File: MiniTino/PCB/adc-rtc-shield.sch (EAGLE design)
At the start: 51 parts, among them IC1 TLC2543, IC2 RV_3049_C2

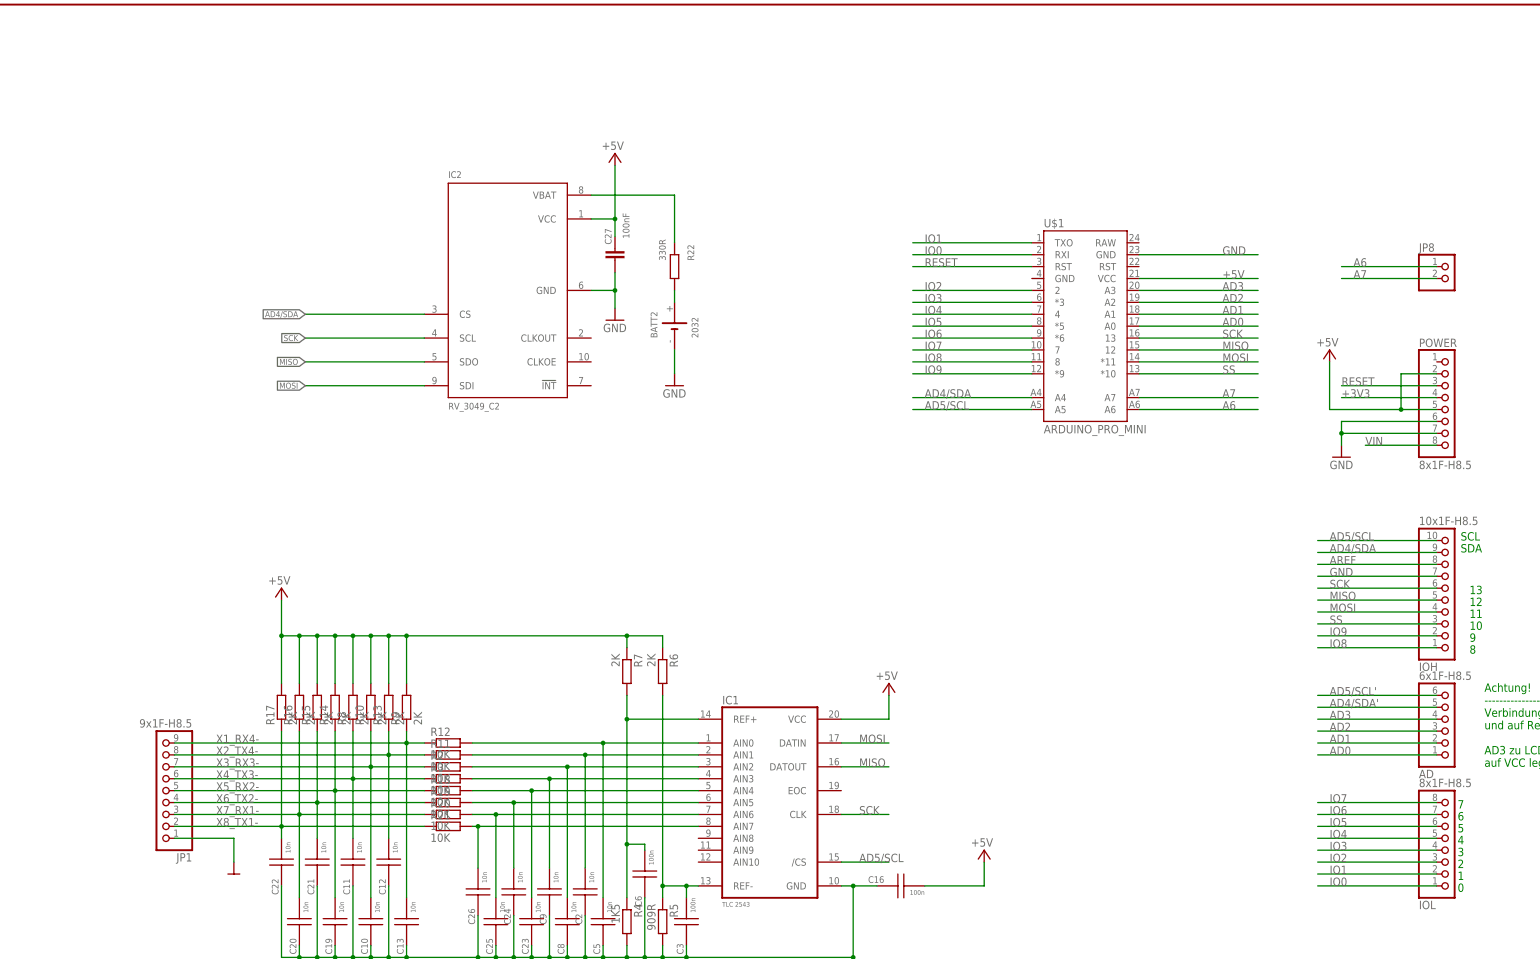
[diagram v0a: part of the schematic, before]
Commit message: Start routing.
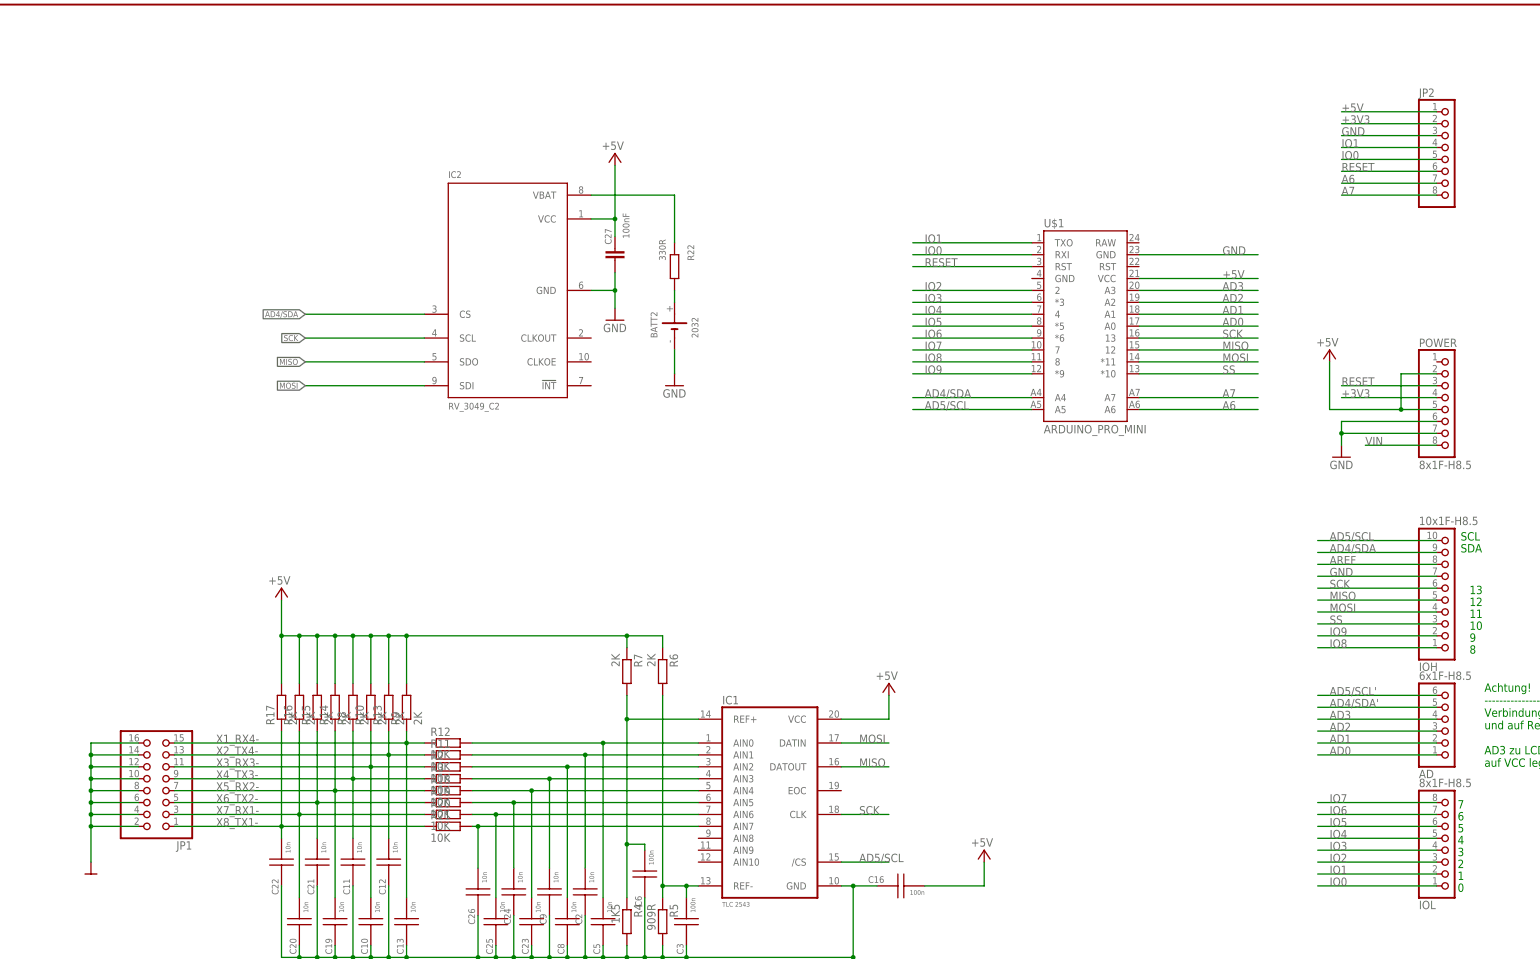
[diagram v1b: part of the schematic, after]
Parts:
- removed JP8: (no value), pinhead:PINHD-1X2
- added JP2: (no value), pinhead:PINHD-1X8/90
- JP1: value 9x1F-H8.5 -> (none); device pinhead:PINHD-1X9/90 -> pinhead:PINHD-2X8/90
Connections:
- net +3V3: now also JP2.2
- net +5V: now also JP2.1
- net A6: now also JP2.7; no longer JP8.1
- net A7: now also JP2.8; no longer JP8.2
- net GND: now also JP1.10, JP1.12, JP1.14, JP1.16, JP1.2, JP1.4, JP1.6, JP1.8, JP2.3; no longer JP1.1
- net IO0: now also JP2.5
- net IO1: now also JP2.4
- net RESET: now also JP2.6
- net X1_RX4-: now also JP1.15; no longer JP1.9
- net X2_TX4-: now also JP1.13; no longer JP1.8
- net X3_RX3-: now also JP1.11; no longer JP1.7
- net X4_TX3-: now also JP1.9; no longer JP1.6
- net X5_RX2-: now also JP1.7; no longer JP1.5
- net X6_TX2-: now also JP1.5; no longer JP1.4
- net X8_TX1-: now also JP1.1; no longer JP1.2
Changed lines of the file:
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@@
 <part name="P+3" library="supply1" deviceset="+5V" device=""/>
 <part name="P+5" library="supply1" deviceset="+5V" device=""/>
-<part name="JP1" library="pinhead" deviceset="PINHD-1X9" device="/90" value="9x1F-H8.5"/>
 <part name="U$1" library="SparkFun-Boards" deviceset="ARDUINO_PRO_MINI" device=""/>
-<part name="JP8" library="pinhead" deviceset="PINHD-1X2" device=""/>
+<part name="JP1" library="pinhead" deviceset="PINHD-2X8" device="/90"/>
+<part name="JP2" library="pinhead" deviceset="PINHD-1X8" device="/90"/>
 </parts>
 <sheets>
@@
 <instance part="R21" gate="G$1" x="116.84" y="88.9"/>
 <instance part="U$5" gate="G$1" x="203.2" y="55.88"/>
-<instance part="U$7" gate="G$1" x="71.12" y="78.74"/>
+<instance part="U$7" gate="G$1" x="40.64" y="78.74"/>
 <instance part="IC2" gate="A" x="129.54" y="203.2"/>
 <instance part="R22" gate="G$1" x="165.1" y="208.28" smashed="yes" rot="MR90">
@@
 <attribute name="VALUE" x="212.725" y="121.92" size="1.778" layer="96" rot="R180"/>
 </instance>
+<instance part="U$1" gate="G$1" x="251.46" y="198.12"/>
 <instance part="JP1" gate="A" x="55.88" y="96.52" rot="R180"/>
-<instance part="U$1" gate="G$1" x="251.46" y="198.12"/>
-<instance part="JP8" gate="G$1" x="330.2" y="205.74"/>
+<instance part="JP2" gate="A" x="330.2" y="231.14"/>
 </instances>
 <busses>
@@
 <junction x="320.04" y="177.8"/>
 <pinref part="U$1" gate="G$1" pin="VCC"/>
+<wire x1="327.66" y1="241.3" x2="307.34" y2="241.3" width="0.1524" layer="91"/>
+<label x="307.34" y="241.3" size="1.778" layer="95"/>
+<pinref part="JP2" gate="A" pin="1"/>
 </segment>
 <segment>
@@
 <pinref part="POWER" gate="A" pin="6"/>
 <pinref part="POWER" gate="A" pin="7"/>
+<wire x1="327.66" y1="236.22" x2="307.34" y2="236.22" width="0.1524" layer="91"/>
+<label x="307.34" y="236.22" size="1.778" layer="95"/>
+<pinref part="JP2" gate="A" pin="3"/>
 </segment>
 <segment>
@@
 <segment>
 <pinref part="U$7" gate="G$1" pin="GND"/>
-<wire x1="58.42" y1="86.36" x2="71.12" y2="86.36" width="0.1524" layer="91"/>
-<wire x1="71.12" y1="86.36" x2="71.12" y2="81.28" width="0.1524" layer="91"/>
-<pinref part="JP1" gate="A" pin="1"/>
+<wire x1="50.8" y1="106.68" x2="40.64" y2="106.68" width="0.1524" layer="91"/>
+<wire x1="40.64" y1="106.68" x2="40.64" y2="104.14" width="0.1524" layer="91"/>
+<wire x1="40.64" y1="104.14" x2="40.64" y2="101.6" width="0.1524" layer="91"/>
+<wire x1="40.64" y1="101.6" x2="40.64" y2="99.06" width="0.1524" layer="91"/>
+<wire x1="40.64" y1="99.06" x2="40.64" y2="96.52" width="0.1524" layer="91"/>
+<wire x1="40.64" y1="96.52" x2="40.64" y2="93.98" width="0.1524" layer="91"/>
+<wire x1="40.64" y1="93.98" x2="40.64" y2="91.44" width="0.1524" layer="91"/>
+<wire x1="40.64" y1="91.44" x2="40.64" y2="88.9" width="0.1524" layer="91"/>
+<wire x1="40.64" y1="88.9" x2="40.64" y2="81.28" width="0.1524" layer="91"/>
+<wire x1="50.8" y1="91.44" x2="40.64" y2="91.44" width="0.1524" layer="91"/>
+<wire x1="50.8" y1="93.98" x2="40.64" y2="93.98" width="0.1524" layer="91"/>
+<wire x1="50.8" y1="96.52" x2="40.64" y2="96.52" width="0.1524" layer="91"/>
+<wire x1="50.8" y1="99.06" x2="40.64" y2="99.06" width="0.1524" layer="91"/>
+<wire x1="50.8" y1="101.6" x2="40.64" y2="101.6" width="0.1524" layer="91"/>
+<wire x1="50.8" y1="104.14" x2="40.64" y2="104.14" width="0.1524" layer="91"/>
+<junction x="40.64" y="104.14"/>
+<junction x="40.64" y="101.6"/>
+<junction x="40.64" y="99.06"/>
+<junction x="40.64" y="96.52"/>
+<junction x="40.64" y="93.98"/>
+<junction x="40.64" y="91.44"/>
+<wire x1="50.8" y1="88.9" x2="40.64" y2="88.9" width="0.1524" layer="91"/>
+<junction x="40.64" y="88.9"/>
+<pinref part="JP1" gate="A" pin="2"/>
+<pinref part="JP1" gate="A" pin="4"/>
+<pinref part="JP1" gate="A" pin="6"/>
+<pinref part="JP1" gate="A" pin="8"/>
+<pinref part="JP1" gate="A" pin="10"/>
+<pinref part="JP1" gate="A" pin="12"/>
+<pinref part="JP1" gate="A" pin="14"/>
+<pinref part="JP1" gate="A" pin="16"/>
 </segment>
 </net>
@@
 <label x="307.34" y="180.34" size="1.778" layer="95"/>
 <pinref part="POWER" gate="A" pin="4"/>
+<wire x1="327.66" y1="238.76" x2="307.34" y2="238.76" width="0.1524" layer="91"/>
+<label x="307.34" y="238.76" size="1.778" layer="95"/>
+<pinref part="JP2" gate="A" pin="2"/>
 </segment>
 </net>
@@
 <label x="218.44" y="213.36" size="1.778" layer="95"/>
 <pinref part="U$1" gate="G$1" pin="TXO"/>
+<wire x1="307.34" y1="233.68" x2="327.66" y2="233.68" width="0.1524" layer="91"/>
+<label x="307.34" y="233.68" size="1.778" layer="95"/>
+<pinref part="JP2" gate="A" pin="4"/>
 </segment>
 </net>
@@
 <label x="218.44" y="210.82" size="1.778" layer="95"/>
 <pinref part="U$1" gate="G$1" pin="RXI"/>
+<wire x1="327.66" y1="231.14" x2="307.34" y2="231.14" width="0.1524" layer="91"/>
+<label x="307.34" y="231.14" size="1.778" layer="95"/>
+<pinref part="JP2" gate="A" pin="5"/>
 </segment>
 </net>
@@
 <pinref part="C12" gate="G$1" pin="2"/>
 <wire x1="58.42" y1="104.14" x2="104.14" y2="104.14" width="0.1524" layer="91"/>
-<pinref part="JP1" gate="A" pin="8"/>
+<pinref part="JP1" gate="A" pin="13"/>
 </segment>
 </net>
@@
 <pinref part="C13" gate="G$1" pin="2"/>
 <wire x1="58.42" y1="106.68" x2="107.95" y2="106.68" width="0.1524" layer="91"/>
-<pinref part="JP1" gate="A" pin="9"/>
+<pinref part="JP1" gate="A" pin="15"/>
 </segment>
 </net>
@@
 <pinref part="C11" gate="G$1" pin="2"/>
 <wire x1="58.42" y1="99.06" x2="96.52" y2="99.06" width="0.1524" layer="91"/>
-<pinref part="JP1" gate="A" pin="6"/>
+<pinref part="JP1" gate="A" pin="9"/>
 </segment>
 </net>
@@
 <pinref part="C10" gate="G$1" pin="2"/>
 <wire x1="58.42" y1="101.6" x2="100.33" y2="101.6" width="0.1524" layer="91"/>
-<pinref part="JP1" gate="A" pin="7"/>
+<pinref part="JP1" gate="A" pin="11"/>
 </segment>
 </net>
@@
 <pinref part="C22" gate="G$1" pin="2"/>
 <pinref part="R21" gate="G$1" pin="1"/>
-<pinref part="JP1" gate="A" pin="2"/>
+<pinref part="JP1" gate="A" pin="1"/>
 </segment>
 </net>
@@
 <pinref part="R15" gate="G$1" pin="1"/>
 <pinref part="R19" gate="G$1" pin="1"/>
-<pinref part="JP1" gate="A" pin="4"/>
+<pinref part="JP1" gate="A" pin="5"/>
 </segment>
 </net>
@@
 <pinref part="C19" gate="G$1" pin="2"/>
 <pinref part="R18" gate="G$1" pin="1"/>
-<pinref part="JP1" gate="A" pin="5"/>
+<pinref part="JP1" gate="A" pin="7"/>
 </segment>
 </net>
@@
 <label x="218.44" y="208.28" size="1.778" layer="95"/>
 <pinref part="U$1" gate="G$1" pin="RST"/>
+<wire x1="327.66" y1="228.6" x2="307.34" y2="228.6" width="0.1524" layer="91"/>
+<label x="307.34" y="228.6" size="1.778" layer="95"/>
+<pinref part="JP2" gate="A" pin="6"/>
 </segment>
 </net>
 <net name="A6" class="0">
 <segment>
-<pinref part="JP8" gate="G$1" pin="1"/>
-<wire x1="327.66" y1="208.28" x2="307.34" y2="208.28" width="0.1524" layer="91"/>
-<label x="309.88" y="208.28" size="1.778" layer="95"/>
+<wire x1="327.66" y1="226.06" x2="307.34" y2="226.06" width="0.1524" layer="91"/>
+<label x="307.34" y="226.06" size="1.778" layer="95"/>
 <wire x1="289.56" y1="177.8" x2="264.16" y2="177.8" width="0.1524" layer="91"/>
 <label x="281.94" y="177.8" size="1.778" layer="95"/>
 <pinref part="U$1" gate="G$1" pin="A6"/>
+<pinref part="JP2" gate="A" pin="7"/>
 </segment>
 </net>
 <net name="A7" class="0">
 <segment>
-<pinref part="JP8" gate="G$1" pin="2"/>
-<wire x1="327.66" y1="205.74" x2="307.34" y2="205.74" width="0.1524" layer="91"/>
-<label x="309.88" y="205.74" size="1.778" layer="95"/>
+<wire x1="327.66" y1="223.52" x2="307.34" y2="223.52" width="0.1524" layer="91"/>
+<label x="307.34" y="223.52" size="1.778" layer="95"/>
 <wire x1="289.56" y1="180.34" x2="264.16" y2="180.34" width="0.1524" layer="91"/>
 <label x="281.94" y="180.34" size="1.778" layer="95"/>
 <pinref part="U$1" gate="G$1" pin="A7"/>
-</segment>
-</net>
+<pinref part="JP2" gate="A" pin="8"/>
+</segment>
+</net>
